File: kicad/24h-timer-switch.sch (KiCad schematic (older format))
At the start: 13 parts, among them J1 Barrel_Jack, J2 Screw_Terminal_01x02, Q1 AO4620, SW1 SW_SPST, U1 AMS1117-5.0, U2 ATtiny85-20PU

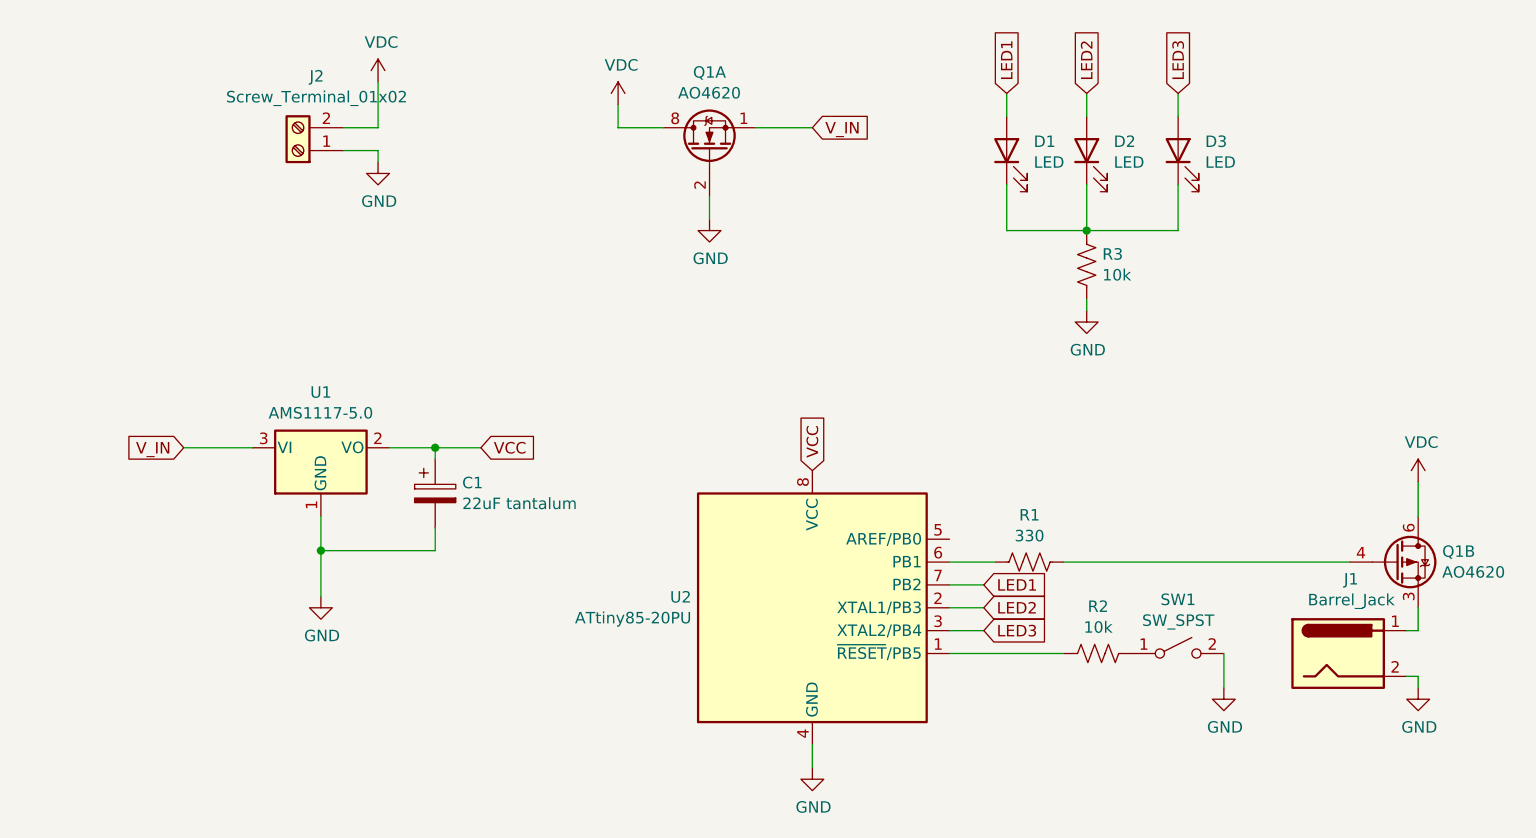
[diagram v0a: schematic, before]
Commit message: full-board
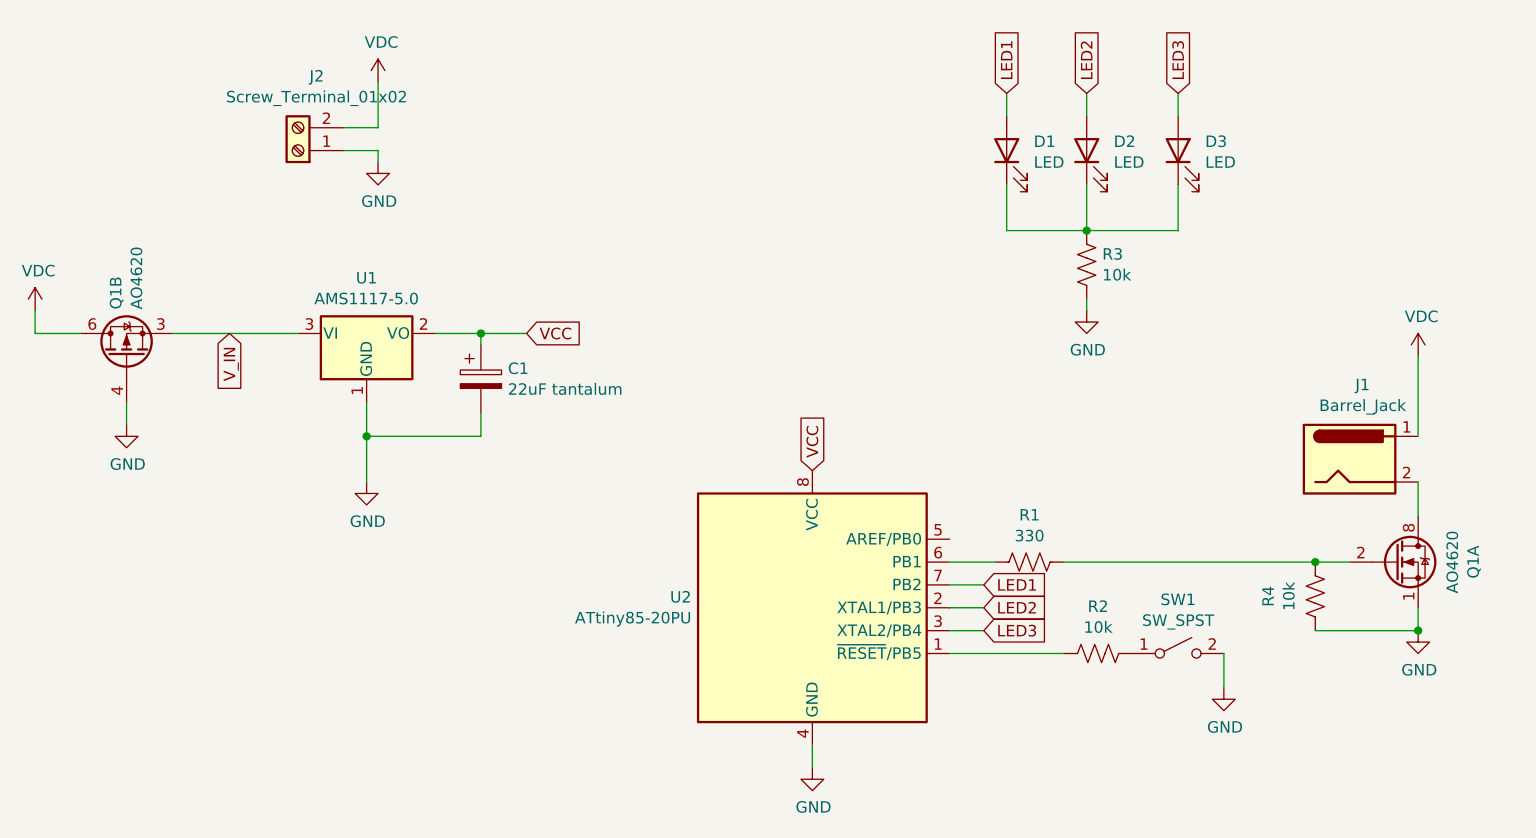
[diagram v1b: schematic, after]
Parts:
- added R4: 10k, Resistor_THT:R_Axial_DIN0207_L6.3mm_D2.5mm_P2.54mm_Vertical, symbol Device:R_US
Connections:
- net GND: now also Q1.1 (S), Q1.4 (G), R4.2; no longer J1.2, Q1.2 (G)
- net VDC: now also J1.1; no longer Q1.7 (D), Q1.8 (D)
- net V_IN: now also Q1.3 (1); no longer Q1.1 (S)
- net at R1.1: now also Q1.2 (G), R4.1; no longer Q1.4 (G)
- new net: J1.2, Q1.7 (D), Q1.8 (D)
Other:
- moved on the sheet: C1, J1, Q1A, Q1B, U1
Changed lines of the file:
@@
 L Regulator_Linear:AMS1117-5.0 U1
 U 1 1 61A27784
-P 2200 2650
-F 0 "U1" H 2200 2892 50  0000 C CNN
-F 1 "AMS1117-5.0" H 2200 2801 50  0000 C CNN
-F 2 "Package_TO_SOT_SMD:SOT-223-3_TabPin2" H 2200 2850 50  0001 C CNN
-F 3 "http://www.advanced-monolithic.com/pdf/ds1117.pdf" H 2300 2400 50  0001 C CNN
-	1    2200 2650
+P 2400 2150
+F 0 "U1" H 2400 2392 50  0000 C CNN
+F 1 "AMS1117-5.0" H 2400 2301 50  0000 C CNN
+F 2 "Package_TO_SOT_SMD:SOT-223-3_TabPin2" H 2400 2350 50  0001 C CNN
+F 3 "http://www.advanced-monolithic.com/pdf/ds1117.pdf" H 2500 1900 50  0001 C CNN
+	1    2400 2150
 	1    0    0    -1
 $EndComp
@@
 L Transistor_FET:FDS4559 Q1
 U 2 1 61A2EE27
+P 1350 2250
+F 0 "Q1" H 1555 2296 50  0000 L CNN
+F 1 "AO4620" H 1555 2205 50  0000 L CNN
+F 2 "Package_SO:SOIC-8_3.9x4.9mm_P1.27mm" H 1550 2175 50  0001 L CNN
+F 3 "https://www.onsemi.com/pub/Collateral/FDS4559-D.PDF" H 1450 2250 50  0001 L CNN
+	2    1350 2250
+	0    -1   -1   0
+$EndComp
+$Comp
+L Transistor_FET:FDS4559 Q1
+U 1 1 61A30ED2
 P 6900 3150
-F 0 "Q1" H 7105 3196 50  0000 L CNN
-F 1 "AO4620" H 7105 3105 50  0000 L CNN
+F 0 "Q1" V 7242 3150 50  0000 C CNN
+F 1 "AO4620" V 7151 3150 50  0000 C CNN
 F 2 "Package_SO:SOIC-8_3.9x4.9mm_P1.27mm" H 7100 3075 50  0001 L CNN
 F 3 "https://www.onsemi.com/pub/Collateral/FDS4559-D.PDF" H 7000 3150 50  0001 L CNN
-	2    6900 3150
-	1    0    0    -1
-$EndComp
-$Comp
-L Transistor_FET:FDS4559 Q1
-U 1 1 61A30ED2
-P 3900 1350
-F 0 "Q1" V 4242 1350 50  0000 C CNN
-F 1 "AO4620" V 4151 1350 50  0000 C CNN
-F 2 "Package_SO:SOIC-8_3.9x4.9mm_P1.27mm" H 4100 1275 50  0001 L CNN
-F 3 "https://www.onsemi.com/pub/Collateral/FDS4559-D.PDF" H 4000 1350 50  0001 L CNN
-	1    3900 1350
-	0    -1   -1   0
+	1    6900 3150
+	1    0    0    -1
 $EndComp
 $Comp
@@
 L Connector:Barrel_Jack J1
 U 1 1 61A3AC29
-P 6650 3550
-F 0 "J1" H 6707 3875 50  0000 C CNN
-F 1 "Barrel_Jack" H 6707 3784 50  0000 C CNN
-F 2 "Connector_BarrelJack:BarrelJack_Horizontal" H 6700 3510 50  0001 C CNN
-F 3 "~" H 6700 3510 50  0001 C CNN
-	1    6650 3550
+P 6700 2700
+F 0 "J1" H 6757 3025 50  0000 C CNN
+F 1 "Barrel_Jack" H 6757 2934 50  0000 C CNN
+F 2 "Connector_BarrelJack:BarrelJack_Horizontal" H 6750 2660 50  0001 C CNN
+F 3 "~" H 6750 2660 50  0001 C CNN
+	1    6700 2700
 	1    0    0    -1
 $EndComp
@@
 Wire Wire Line
 	2450 1350 2300 1350
-$Comp
-L power:GND #PWR010
-U 1 1 61A3FEB1
-P 7000 3700
-F 0 "#PWR010" H 7000 3450 50  0001 C CNN
-F 1 "GND" H 7005 3527 50  0000 C CNN
-F 2 "" H 7000 3700 50  0001 C CNN
-F 3 "" H 7000 3700 50  0001 C CNN
-	1    7000 3700
-	1    0    0    -1
-$EndComp
-Wire Wire Line
-	3500 1150 3500 1250
-Wire Wire Line
-	3500 1250 3700 1250
+Wire Wire Line
+	950  2050 950  2150
+Wire Wire Line
+	950  2150 1150 2150
 $Comp
 L power:GND #PWR05
 U 1 1 61A42EA9
-P 3900 1650
-F 0 "#PWR05" H 3900 1400 50  0001 C CNN
-F 1 "GND" H 3905 1477 50  0000 C CNN
-F 2 "" H 3900 1650 50  0001 C CNN
-F 3 "" H 3900 1650 50  0001 C CNN
-	1    3900 1650
-	1    0    0    -1
-$EndComp
-Wire Wire Line
-	3900 1550 3900 1650
-Wire Wire Line
-	4100 1250 4350 1250
-Text GLabel 4350 1250 2    50   Input ~ 0
-V_IN
-Wire Wire Line
-	1900 2650 1600 2650
-Text GLabel 1600 2650 0    50   Input ~ 0
+P 1350 2550
+F 0 "#PWR05" H 1350 2300 50  0001 C CNN
+F 1 "GND" H 1355 2377 50  0000 C CNN
+F 2 "" H 1350 2550 50  0001 C CNN
+F 3 "" H 1350 2550 50  0001 C CNN
+	1    1350 2550
+	1    0    0    -1
+$EndComp
+Wire Wire Line
+	1350 2450 1350 2550
+Text GLabel 1800 2150 3    50   Input ~ 0
 V_IN
 $Comp
 L power:GND #PWR01
 U 1 1 61A444A1
-P 2200 3300
-F 0 "#PWR01" H 2200 3050 50  0001 C CNN
-F 1 "GND" H 2205 3127 50  0000 C CNN
-F 2 "" H 2200 3300 50  0001 C CNN
-F 3 "" H 2200 3300 50  0001 C CNN
-	1    2200 3300
-	1    0    0    -1
-$EndComp
-Wire Wire Line
-	2200 2950 2200 3100
+P 2400 2800
+F 0 "#PWR01" H 2400 2550 50  0001 C CNN
+F 1 "GND" H 2405 2627 50  0000 C CNN
+F 2 "" H 2400 2800 50  0001 C CNN
+F 3 "" H 2400 2800 50  0001 C CNN
+	1    2400 2800
+	1    0    0    -1
+$EndComp
+Wire Wire Line
+	2400 2450 2400 2600
 $Comp
 L Device:CP C1
 U 1 1 61A472D0
-P 2700 2850
-F 0 "C1" H 2818 2896 50  0000 L CNN
-F 1 "22uF tantalum" H 2818 2805 50  0000 L CNN
-F 2 "Capacitor_THT:CP_Radial_D5.0mm_P2.50mm" H 2738 2700 50  0001 C CNN
-F 3 "~" H 2700 2850 50  0001 C CNN
-	1    2700 2850
-	1    0    0    -1
-$EndComp
-Wire Wire Line
-	2500 2650 2700 2650
-Wire Wire Line
-	2700 2650 2700 2700
-Wire Wire Line
-	2700 3000 2700 3100
-Wire Wire Line
-	2700 3100 2200 3100
-Wire Wire Line
-	2200 3100 2200 3300
-Connection ~ 2200 3100
+P 2900 2350
+F 0 "C1" H 3018 2396 50  0000 L CNN
+F 1 "22uF tantalum" H 3018 2305 50  0000 L CNN
+F 2 "Capacitor_THT:CP_Radial_D5.0mm_P2.50mm" H 2938 2200 50  0001 C CNN
+F 3 "~" H 2900 2350 50  0001 C CNN
+	1    2900 2350
+	1    0    0    -1
+$EndComp
+Wire Wire Line
+	2700 2150 2900 2150
+Wire Wire Line
+	2900 2150 2900 2200
+Wire Wire Line
+	2900 2500 2900 2600
+Wire Wire Line
+	2900 2600 2400 2600
+Wire Wire Line
+	2400 2600 2400 2800
+Connection ~ 2400 2600
 $Comp
 L power:VDC #PWR02
@@
 L power:VDC #PWR04
 U 1 1 61A4B547
-P 3500 1150
-F 0 "#PWR04" H 3500 1050 50  0001 C CNN
-F 1 "VDC" H 3515 1323 50  0000 C CNN
-F 2 "" H 3500 1150 50  0001 C CNN
-F 3 "" H 3500 1150 50  0001 C CNN
-	1    3500 1150
-	1    0    0    -1
-$EndComp
-Wire Wire Line
-	2700 2650 2900 2650
-Connection ~ 2700 2650
-Text GLabel 2900 2650 2    50   Input ~ 0
+P 950 2050
+F 0 "#PWR04" H 950 1950 50  0001 C CNN
+F 1 "VDC" H 965 2223 50  0000 C CNN
+F 2 "" H 950 2050 50  0001 C CNN
+F 3 "" H 950 2050 50  0001 C CNN
+	1    950  2050
+	1    0    0    -1
+$EndComp
+Wire Wire Line
+	2900 2150 3100 2150
+Connection ~ 2900 2150
+Text GLabel 3100 2150 2    50   Input ~ 0
 VCC
 Text GLabel 4350 2750 1    50   Input ~ 0
@@
 L power:VDC #PWR09
 U 1 1 61A51849
-P 7000 2800
-F 0 "#PWR09" H 7000 2700 50  0001 C CNN
-F 1 "VDC" H 7015 2973 50  0000 C CNN
-F 2 "" H 7000 2800 50  0001 C CNN
-F 3 "" H 7000 2800 50  0001 C CNN
-	1    7000 2800
+P 7000 2250
+F 0 "#PWR09" H 7000 2150 50  0001 C CNN
+F 1 "VDC" H 7015 2423 50  0000 C CNN
+F 2 "" H 7000 2250 50  0001 C CNN
+F 3 "" H 7000 2250 50  0001 C CNN
+	1    7000 2250
 	1    0    0    -1
 $EndComp
@@
 	7000 2800 7000 2950
 Wire Wire Line
-	5450 3150 6700 3150
+	5450 3150 6550 3150
 $Comp
 L Device:R_US R2
@@
 $EndComp
 Wire Wire Line
+	7000 2250 7000 2600
+Wire Wire Line
 	7000 3350 7000 3450
-Wire Wire Line
-	7000 3450 6950 3450
-Wire Wire Line
-	7000 3700 7000 3650
-Wire Wire Line
-	7000 3650 6950 3650
+$Comp
+L power:GND #PWR010
+U 1 1 61A3FEB1
+P 7000 3450
+F 0 "#PWR010" H 7000 3200 50  0001 C CNN
+F 1 "GND" H 7005 3277 50  0000 C CNN
+F 2 "" H 7000 3450 50  0001 C CNN
+F 3 "" H 7000 3450 50  0001 C CNN
+	1    7000 3450
+	1    0    0    -1
+$EndComp
+$Comp
+L Device:R_US R4
+U 1 1 61C064DB
+P 6550 3300
+F 0 "R4" V 6345 3300 50  0000 C CNN
+F 1 "10k" V 6436 3300 50  0000 C CNN
+F 2 "Resistor_THT:R_Axial_DIN0207_L6.3mm_D2.5mm_P2.54mm_Vertical" V 6590 3290 50  0001 C CNN
+F 3 "~" H 6550 3300 50  0001 C CNN
+	1    6550 3300
+	1    0    0    -1
+$EndComp
+Connection ~ 6550 3150
+Wire Wire Line
+	6550 3150 6700 3150
+Wire Wire Line
+	6550 3450 7000 3450
+Connection ~ 7000 3450
+Wire Wire Line
+	1550 2150 2100 2150
 $EndSCHEMATC
